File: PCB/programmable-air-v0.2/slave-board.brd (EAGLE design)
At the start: 97.7 x 47 mm, 26 parts, among them Q1 600mA/40V, Q2 600mA/40V, Q3 600mA/40V

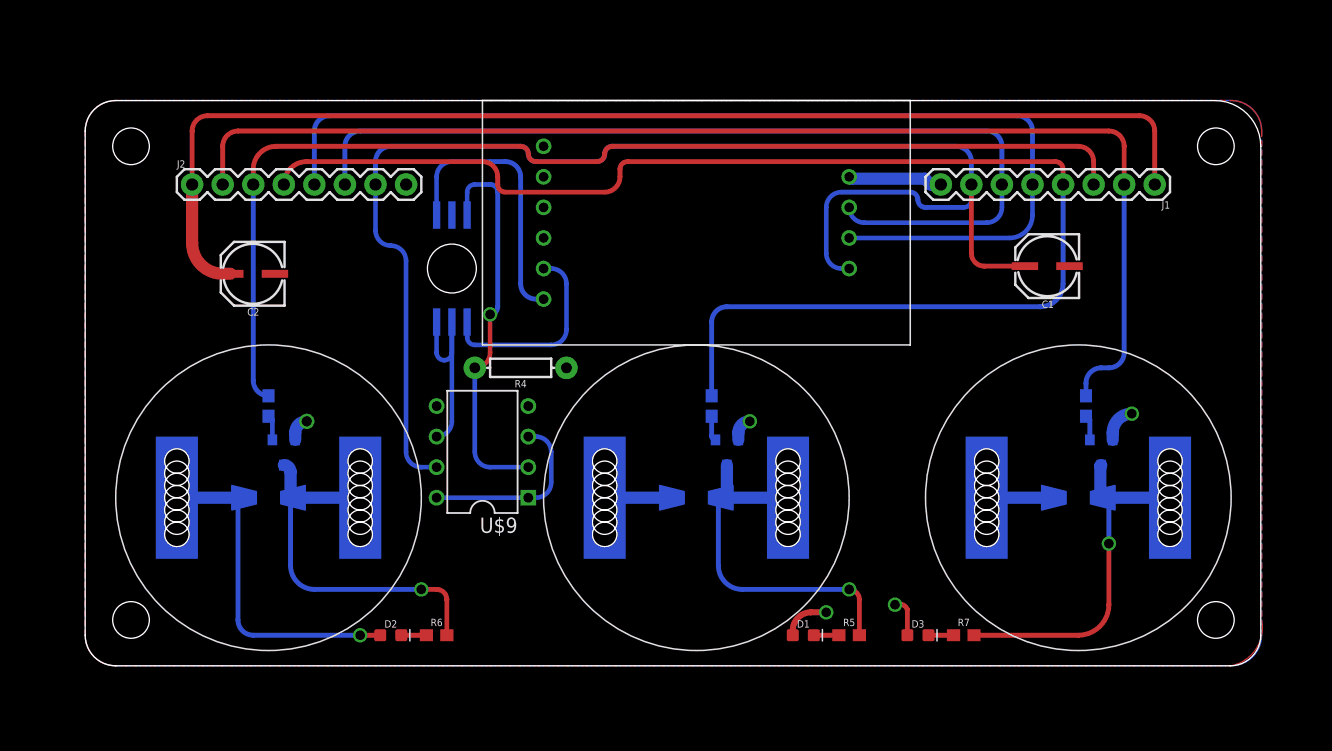
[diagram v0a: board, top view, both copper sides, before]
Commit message: LM358 slave board ready
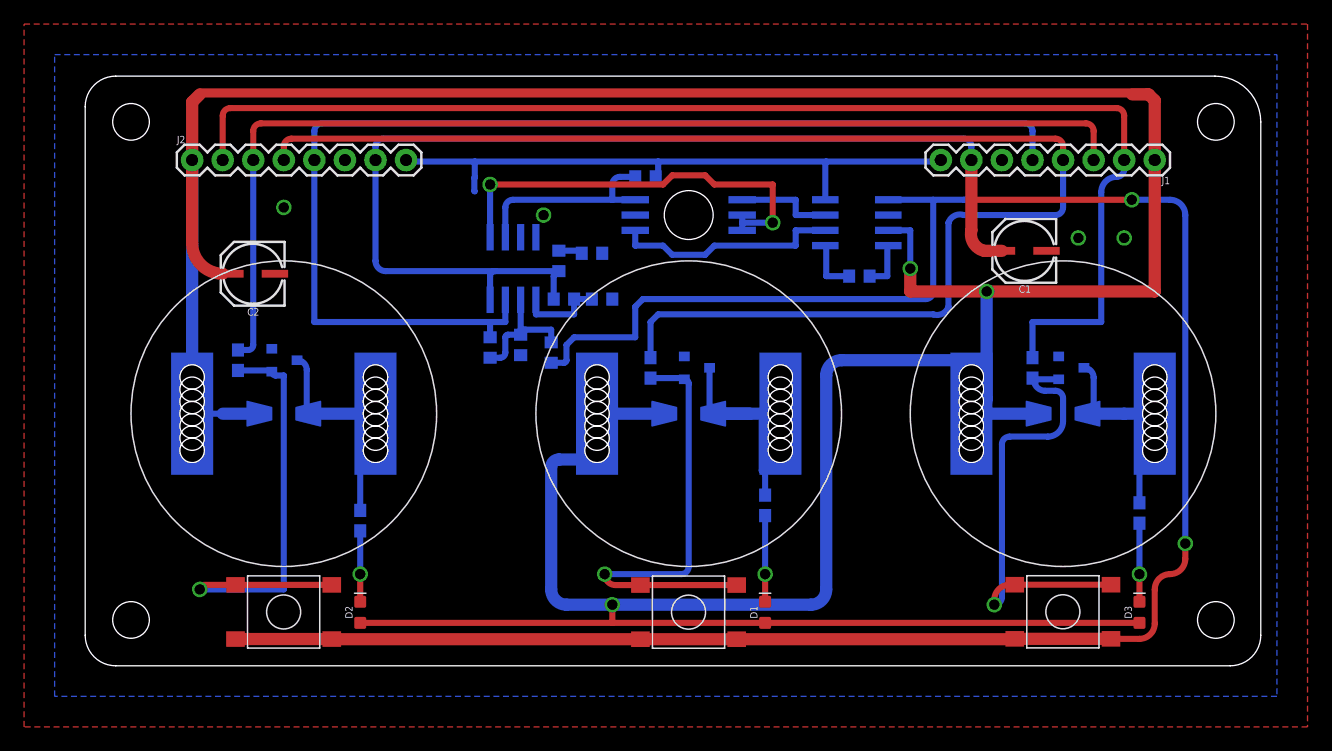
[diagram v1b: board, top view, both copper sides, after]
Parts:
- removed R4: (no value), SparkFun-Resistors:AXIAL-0.3
- added IC1: INA126U, INA126:SO08
- added IC3: LM358MX, linear:SO08
- added R10: 1.78K, eagle-ltspice:R0603
- added R13, R14, R15, R8, R9: 10K, eagle-ltspice:R0603
- added R16: 40K, eagle-ltspice:R0603
- added R17, R20: 20K, eagle-ltspice:R0603
- added U$10: BUTTON, programmable-air-components:BUTTON
- U$1: value HX711 -> 2SMPP-03; device programmable-air-components:HX711 -> programmable-air-components:2SMPP-03
- U$8: value 2SMPP-03 -> BUTTON; device programmable-air-components:2SMPP-03 -> programmable-air-components:BUTTON
- U$9: value LM10CN -> BUTTON; device programmable-air-components:DIP8 -> programmable-air-components:BUTTON
- moved U$8 34.7 mm to (50.1, 4.46), turned to 180 degrees
- moved U$9 21.2 mm to (16.5, 4.47), turned to 180 degrees
- moved D3 18.5 mm to (87.6, 4.45), turned to 90 degrees
- moved R7 17.8 mm to (87.6, 12.7), flipped to the bottom, turned to 90 degrees
- moved R5 12.9 mm to (56.5, 13.3), flipped to the bottom, turned to 90 degrees
- moved R6 11.4 mm to (22.9, 12.1), flipped to the bottom, turned to 90 degrees
- moved Q2 7.62 mm to (16.5, 25.4), turned to 90 degrees
- moved Q1 7.43 mm to (50.8, 24.8), turned to 90 degrees
- moved Q3 7.43 mm to (81.9, 24.8), turned to 90 degrees
- moved U$3 7.10 mm to (16.5, 21.0)
- moved U$6 7.10 mm to (16.5, 21.0)
- moved U$4 7.10 mm to (81.3, 21.0)
- moved U$7 7.10 mm to (81.3, 21.0)
- moved U$2 7.01 mm to (50.2, 21.0)
- moved U$5 7.01 mm to (50.2, 21.0)
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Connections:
- removed net N$16: U$8.P$5, U$8.P$6, U$9.6
- removed net N$17: R4.P$2, U$8.P$3, U$9.2
- removed net N$21: U$1.P$6, U$8.P$1
- removed net N$22: U$1.P$5, U$8.P$4
- new net N$19: IC3.1, U$1.P$5, U$1.P$6
- new net N$20: IC1.3, U$1.P$4
- new net N$24: IC3.3, R16.1, R8.2
- new net N$25: IC1.8, R10.1
- new net N$26: IC1.1, R10.2
- new net N$27: IC3.6, R13.2, R17.2, R20.1
- new net N$30: IC3.5, R14.2, R15.1
- new net N$31: IC3.2, R9.2, U$1.P$3
- net GND: now also IC1.4, IC3.4, R14.1, R17.1, R8.1, R9.1; no longer R4.P$1, U$1.P$7, U$9.4
- net N$1: now also U$8.P$2, U$8.P$4
- net N$13: now also IC3.7, R13.1; no longer U$1.P$9
- net N$14: no longer U$1.P$8
- net N$15: now also IC1.5, IC3.8, R15.2, R16.2, R20.2, U$10.P$1, U$10.P$3, U$8.P$1, U$8.P$3, U$9.P$1, U$9.P$3; no longer U$1.P$10, U$9.7
- net N$2: now also U$9.P$2, U$9.P$4
- net N$3: now also U$10.P$2, U$10.P$4
- net N$4: now also IC1.2, U$1.P$1; no longer U$9.1, U$9.3, U$9.8
- net VIN: now also IC1.7
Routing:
- net VIN: track 146.3 -> 417.3 mm
- net N$15: track 113.3 -> 322.2 mm, vias 0 -> 2
- net N$14: track 77.7 -> 0.00 mm
- net N$2: track 2.09 -> 39.9 mm, vias 0 -> 1
- net GND: track 14.6 -> 51.6 mm, vias 3 -> 4
- net N$19: track 0.00 -> 35.5 mm, vias 0 -> 2
- net N$3: track 2.09 -> 37.3 mm, vias 0 -> 1
- net N$1: track 2.09 -> 37.2 mm, vias 0 -> 1
- net N$17: track 32.3 -> 0.00 mm, vias 1 -> 0
- net N$21: track 22.5 -> 0.00 mm
- net N$31: track 0.00 -> 17.0 mm
- net N$16: track 16.9 -> 0.00 mm
- net N$22: track 16.6 -> 0.00 mm
- net N$8: track 31.5 -> 15.4 mm, vias 1 -> 0
- net N$27: track 0.00 -> 11.9 mm
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- added copper zone on layer 16, net GND
- removed copper zone on layer 16, net VIN
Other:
- board size 97.7 x 47 mm -> 97.7 x 49 mm
